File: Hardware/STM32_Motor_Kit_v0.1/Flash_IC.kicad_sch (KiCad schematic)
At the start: 10 parts, among them U16 M24C64-WMN6TP

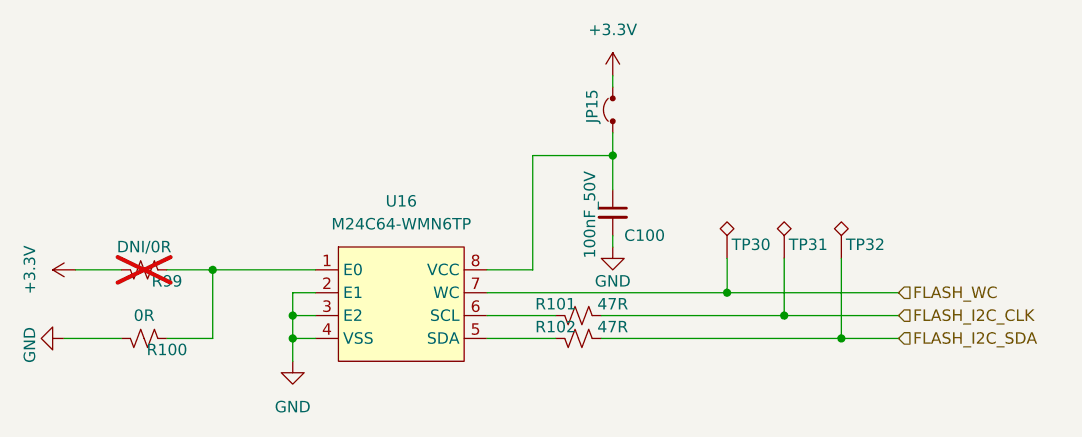
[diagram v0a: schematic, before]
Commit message: 12.01.2025
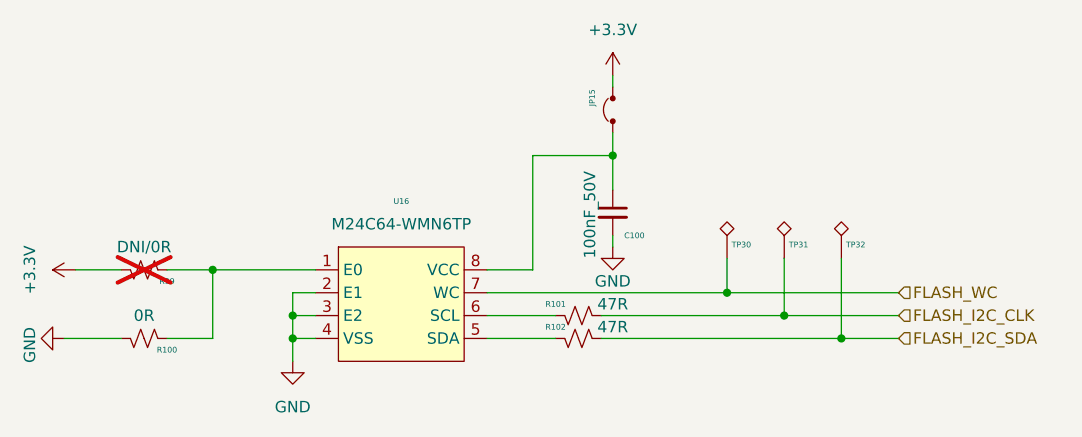
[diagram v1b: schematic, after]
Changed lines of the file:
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@@
 			(effects
 				(font
-					(size 1.27 1.27)
+					(face "Arial")
+					(size 0.635 0.635)
 				)
 			)
@@
 			(effects
 				(font
-					(size 1.27 1.27)
+					(face "Arial")
+					(size 0.635 0.635)
 				)
 				(hide yes)
@@
 			(effects
 				(font
-					(size 1.27 1.27)
+					(face "Arial")
+					(size 0.635 0.635)
 				)
 				(hide yes)
@@
 			(effects
 				(font
-					(size 1.27 1.27)
+					(face "Arial")
+					(size 0.635 0.635)
 				)
 				(hide yes)
@@
 			(effects
 				(font
-					(size 1.27 1.27)
+					(face "Arial")
+					(size 0.635 0.635)
 				)
 				(hide yes)
@@
 			(effects
 				(font
-					(size 1.27 1.27)
+					(face "Arial")
+					(size 0.635 0.635)
 				)
 			)
@@
 			(effects
 				(font
-					(size 1.27 1.27)
+					(face "Arial")
+					(size 0.635 0.635)
 				)
 				(justify left)
@@
 			(effects
 				(font
-					(size 1.27 1.27)
+					(face "Arial")
+					(size 0.635 0.635)
 				)
 				(justify left)
@@
 			(effects
 				(font
-					(size 1.27 1.27)
+					(face "Arial")
+					(size 0.635 0.635)
 				)
 			)
@@
 			(effects
 				(font
-					(size 1.27 1.27)
+					(face "Arial")
+					(size 0.635 0.635)
 				)
 			)
@@
 			(effects
 				(font
-					(size 1.27 1.27)
+					(face "Arial")
+					(size 0.635 0.635)
 				)
 				(justify right)
@@
 			(effects
 				(font
-					(size 1.27 1.27)
+					(face "Arial")
+					(size 0.635 0.635)
 				)
 			)
@@
 			(effects
 				(font
-					(size 1.27 1.27)
+					(face "Arial")
+					(size 0.635 0.635)
 				)
 				(justify left)
@@
 			(effects
 				(font
-					(size 1.27 1.27)
+					(face "Arial")
+					(size 0.635 0.635)
 				)
 				(justify left)
@@
 			(effects
 				(font
-					(size 1.27 1.27)
-				)
-				(hide yes)
+					(face "Arial")
+					(size 0.635 0.635)
+				)
+				(hide yes)

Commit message: Şema üzerinde değişiklikler devam ediyor
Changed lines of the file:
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@@
 (kicad_sch
-	(version 20231120)
+	(version 20250114)
 	(generator "eeschema")
-	(generator_version "8.0")
+	(generator_version "9.0")
 	(paper "A4")
 	(junction
@@
 		(shape input)
 		(at 191.77 78.74 0)
-		(fields_autoplaced yes)
 		(effects
 			(font
@@
 		(shape input)
 		(at 191.77 83.82 0)
-		(fields_autoplaced yes)
 		(effects
 			(font
@@
 		(shape input)
 		(at 191.77 81.28 0)
-		(fields_autoplaced yes)
 		(effects
 			(font
